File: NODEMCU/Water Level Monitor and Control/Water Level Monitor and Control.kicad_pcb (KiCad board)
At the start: 2 copper layers, 123.8 x 85.6 mm, 79 parts, among them J1 12VAC_IN, J2 PUMP, K1 10A RELAY, U1 ESP8266 NODEMCU, U2 HC-SR04, U3 LM2596S-5V, U4 PCA9555D

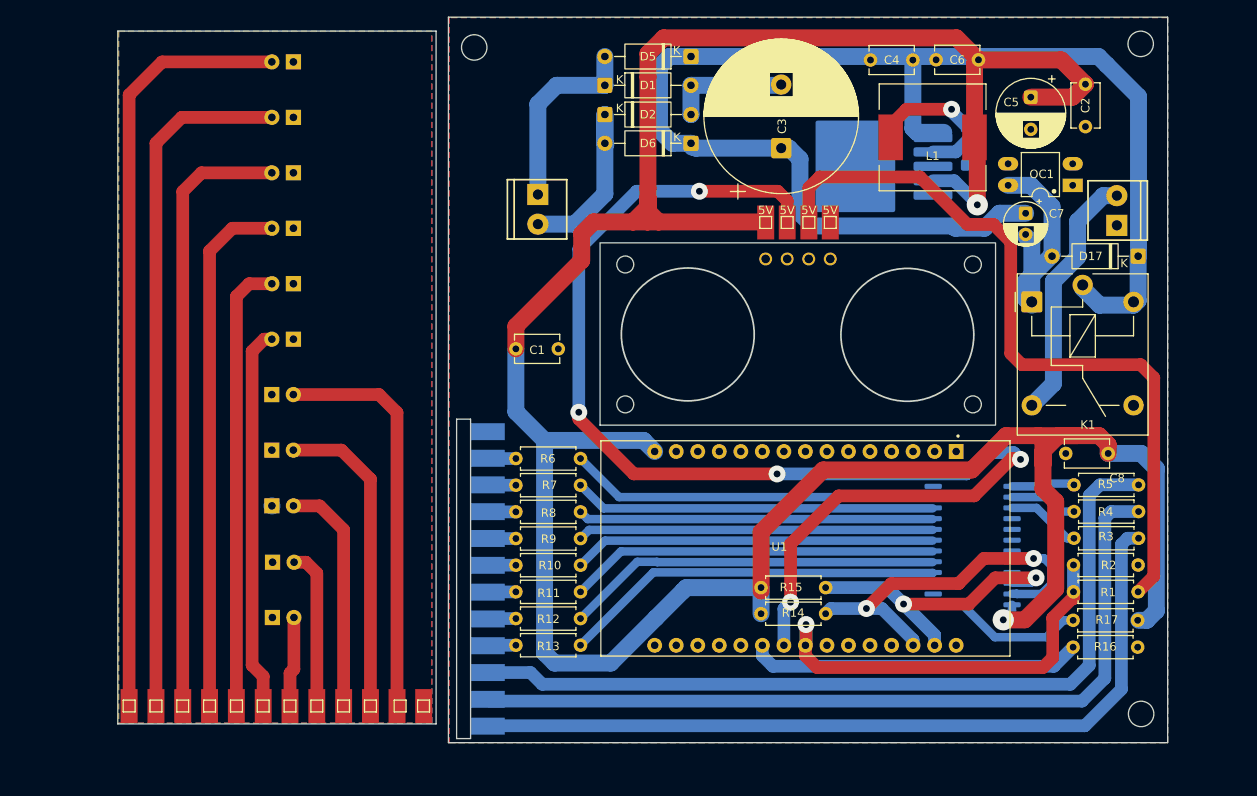
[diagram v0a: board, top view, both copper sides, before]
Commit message: PCB layer ready for printing
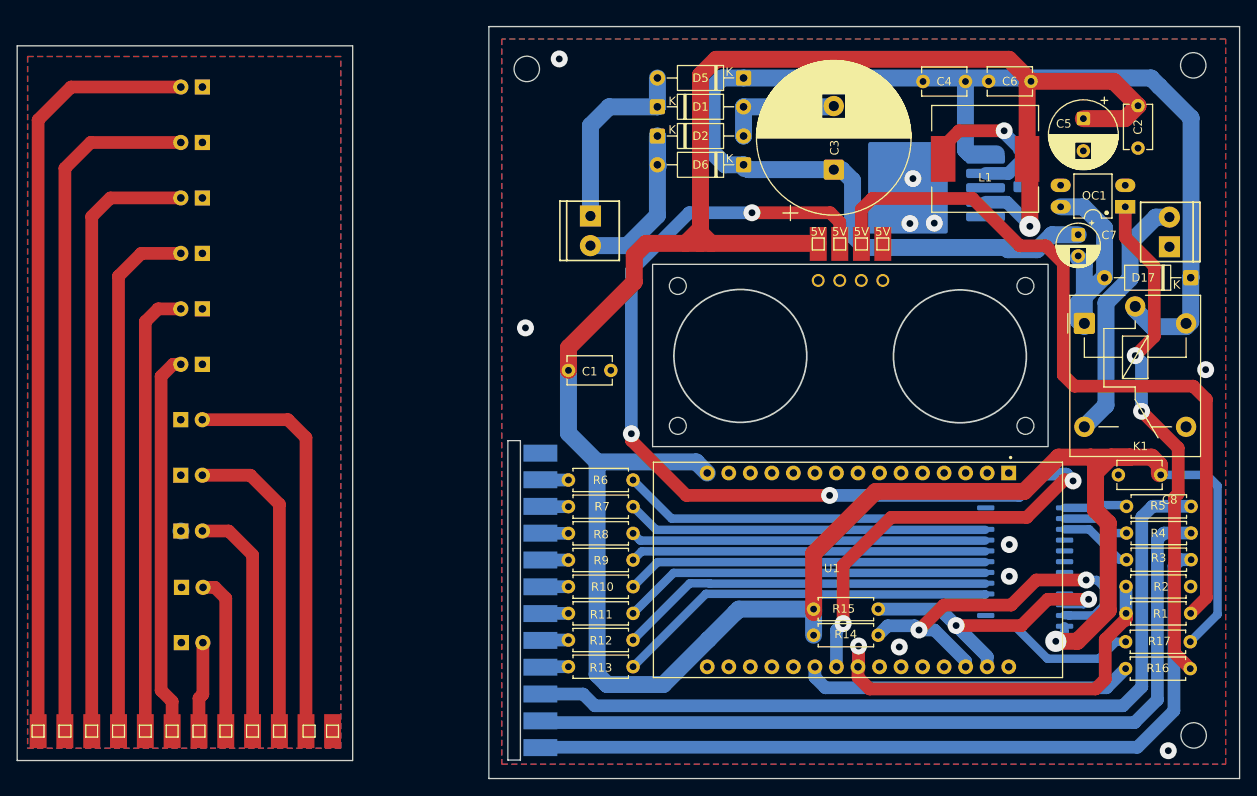
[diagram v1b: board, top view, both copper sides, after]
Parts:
- moved 5V 11.1 mm to (89.7, 141.5)
- moved 5V 11.1 mm to (111.8, 141.5)
- moved 5V 11.1 mm to (99.2, 141.5)
- moved 5V 11.1 mm to (92.8, 141.5)
- moved 5V 11.1 mm to (115.0, 141.5)
- moved 5V 11.1 mm to (105.5, 141.5)
- moved 5V 11.1 mm to (124.4, 141.5)
- moved 5V 11.1 mm to (108.7, 141.5)
- moved 5V 11.1 mm to (102.3, 141.5)
- moved D10 11.1 mm to (106.5, 117.9)
- moved D8 11.1 mm to (106.5, 104.8)
- moved 5V 11.1 mm to (96.0, 141.5)
- moved 5V 11.1 mm to (121.6, 141.5)
- moved 5V 11.1 mm to (118.1, 141.5)
- moved D11 11.1 mm to (106.6, 124.6)
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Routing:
- net Net-(OC1-Pad1): track 0.00 -> 59.9 mm, vias 0 -> 2
- net +5V: track 351.6 -> 352.6 mm
- net GND: vias 0 -> 10
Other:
- board size 123.8 x 85.6 mm -> 144.2 x 88.7 mm
